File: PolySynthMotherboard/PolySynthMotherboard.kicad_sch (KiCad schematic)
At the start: 0 parts

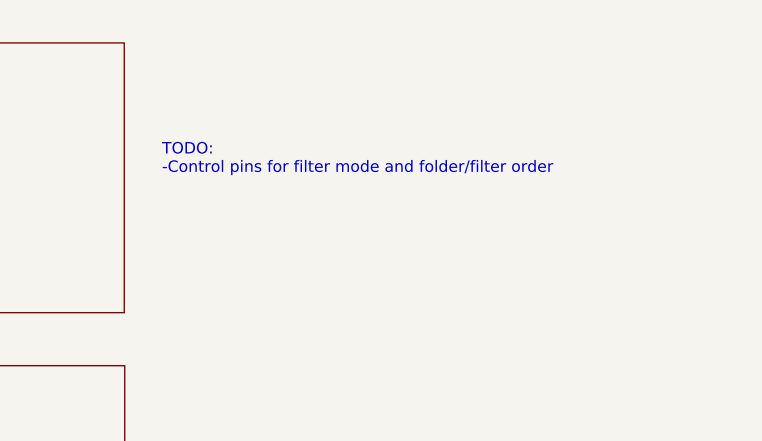
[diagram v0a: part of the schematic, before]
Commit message: power supply tweaks
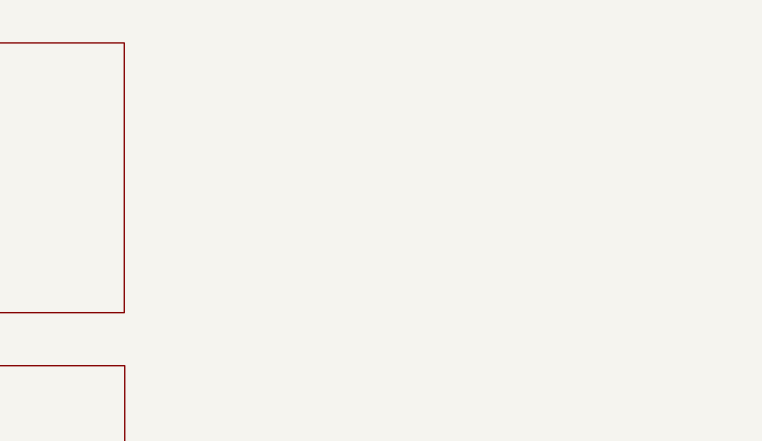
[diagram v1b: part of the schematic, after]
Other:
- note removed: "TODO: -Control pins for filter mode and folder/filter order"
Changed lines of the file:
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@@
 (kicad_sch (version 20230121) (generator eeschema)
   (paper "A4")
-  (text "TODO:\n-Control pins for filter mode and folder/filter order"
-    (at 140.081 32.004 0)
-    (effects (font (size 1.27 1.27)) (justify left bottom))
-  )
   (sheet (at 97.7392 53.1368) (size 38.2016 27.7368) (fields_autoplaced)
     (stroke (width 0.1524) (type solid))
